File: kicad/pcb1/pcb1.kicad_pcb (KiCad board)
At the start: 2 copper layers, 42.5 x 54 mm, 5 parts, among them J1 Conn_01x12_Pin, SW1 SW_Push

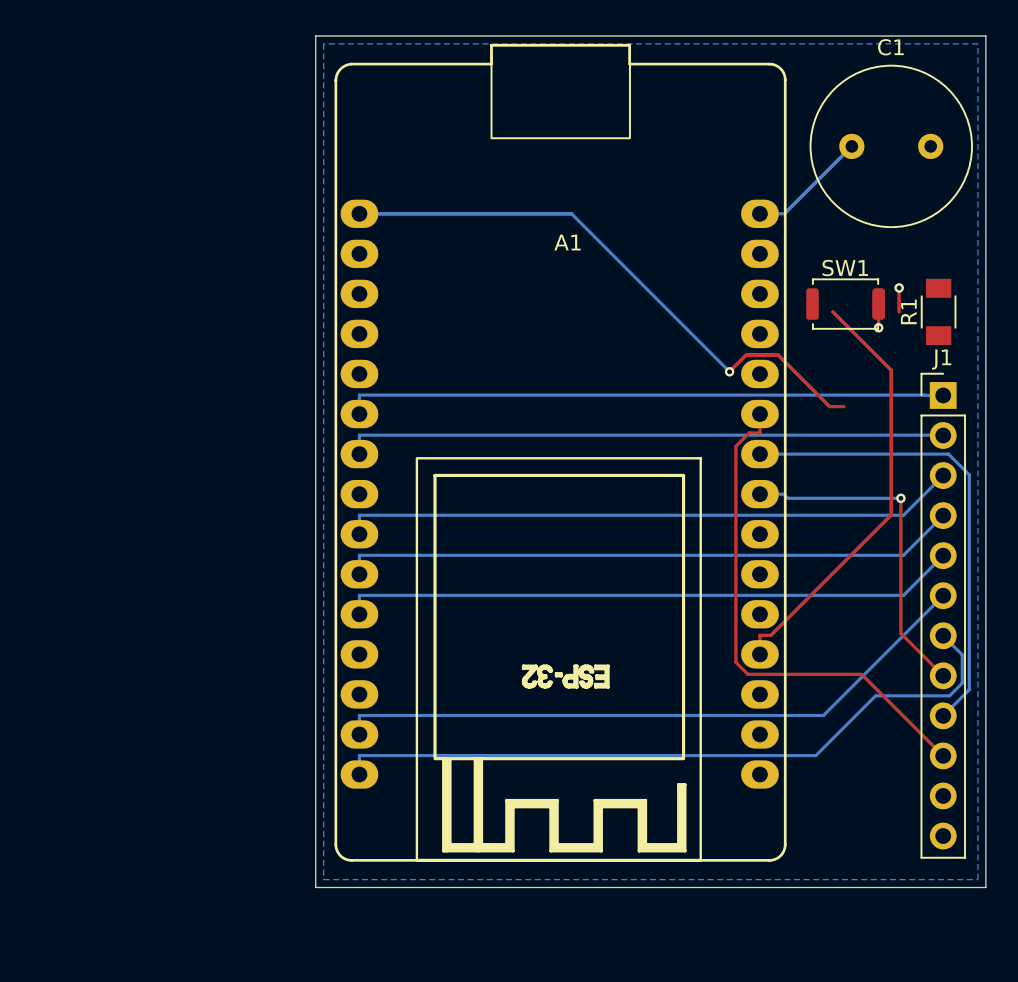
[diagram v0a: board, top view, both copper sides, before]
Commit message: BOM aufgenommen
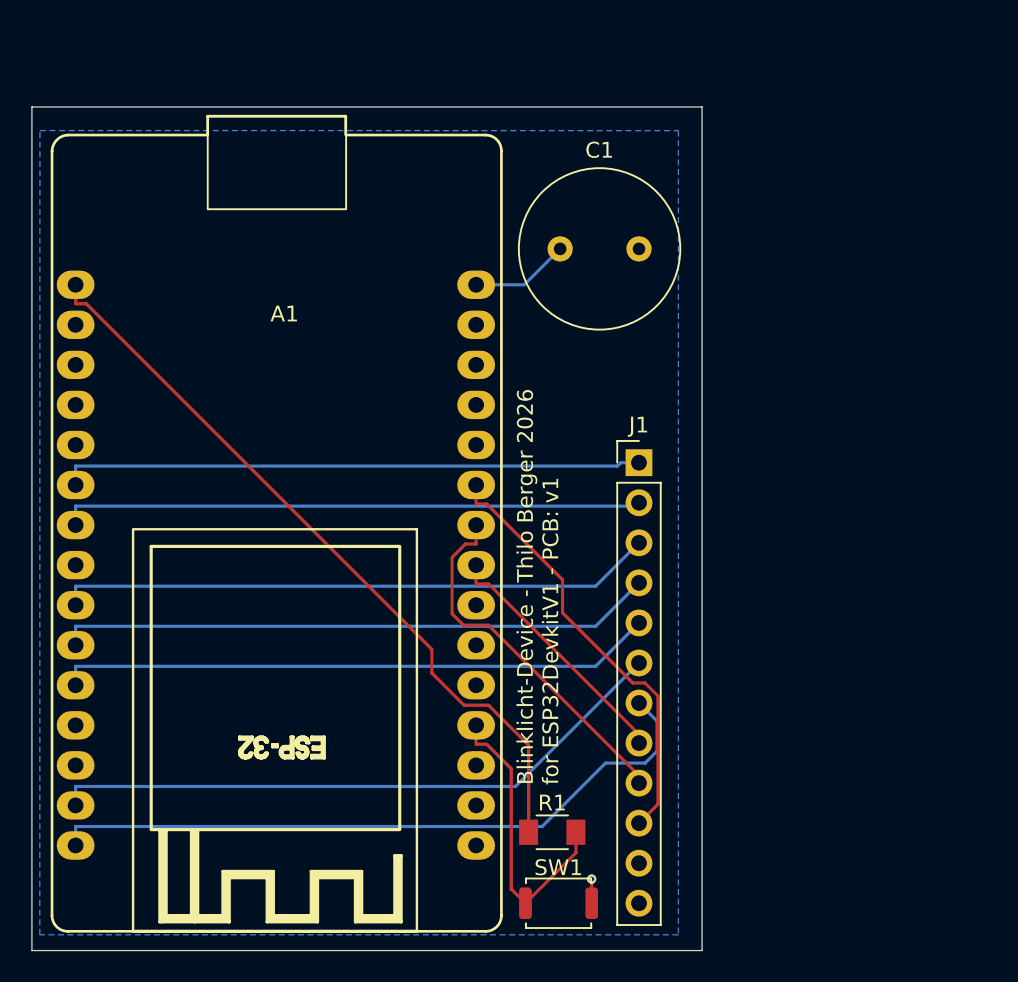
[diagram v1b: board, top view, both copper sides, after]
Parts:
- moved SW1 42.1 mm to (100.4, 115.0)
- moved R1 41.1 mm to (100.0, 110.5), turned to 0 degrees
- moved J1 19.8 mm to (105.5, 87.1)
- moved C1 19.6 mm to (100.5, 73.5)
- moved A1 18.6 mm to (69.8, 75.8)
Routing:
- net Net-(A1-ADC1_CH6/D34): track 53.0 -> 18.8 mm
- net 3V3: track 58.3 -> 47.9 mm, vias 1 -> 0
- net Net-(A1-VIN): track 13.6 -> 6.27 mm
- net D26: track 29.8 -> 23.2 mm
- net D25: track 21.4 -> 16.0 mm, vias 1 -> 0
- net D27: track 32.4 -> 27.6 mm
- net GND: track 3.03 -> 1.53 mm, vias 2 -> 1
- net D23: track 44.8 -> 43.6 mm
- net D17: track 38.2 -> 37.0 mm
- net D16: track 38.2 -> 37.0 mm
- net D22: track 41.4 -> 40.2 mm
- net D21: track 39.3 -> 38.1 mm
- net D19: track 39.3 -> 38.1 mm
- net D18: track 39.3 -> 38.1 mm
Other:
- board size 42.5 x 54 mm -> 42.5 x 53.5 mm
- board text added: "Blinklicht-Device - Thilo Berger 2026 for ESP32DevkitV1 - PCB: v1"
